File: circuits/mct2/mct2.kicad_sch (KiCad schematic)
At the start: 16 parts

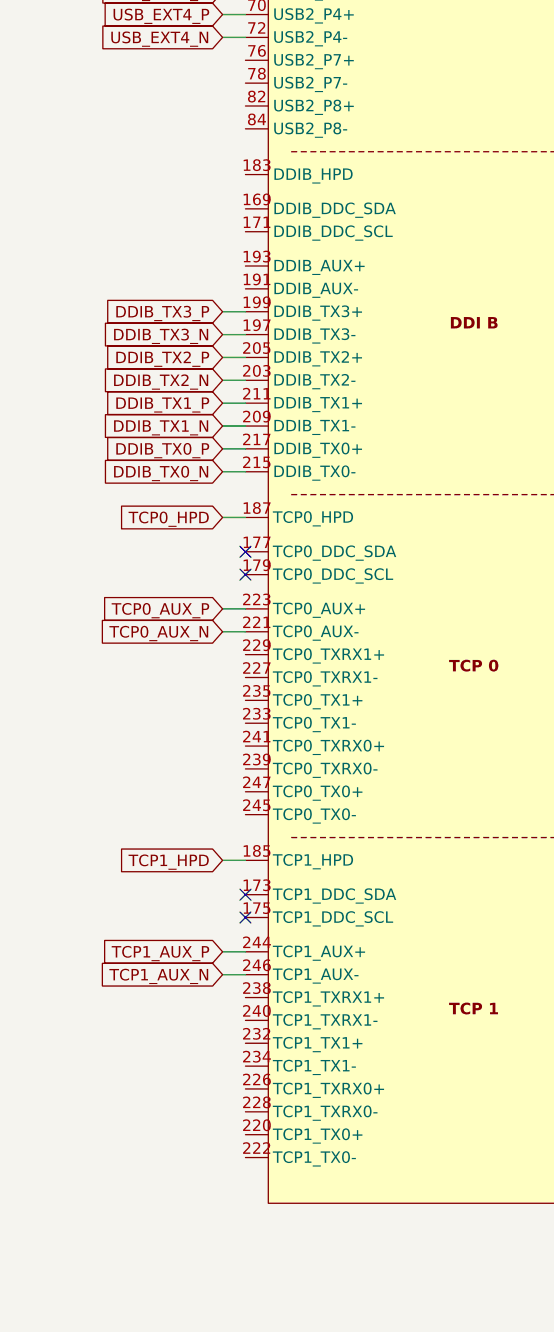
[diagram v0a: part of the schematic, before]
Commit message: Aug 14, 2024 old stuff
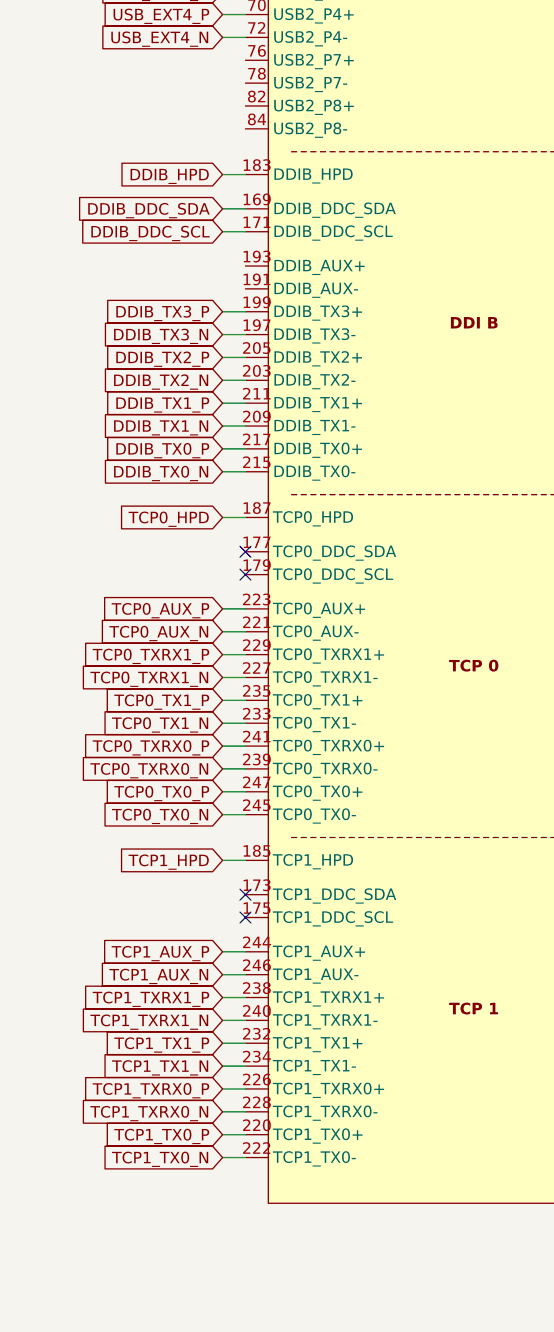
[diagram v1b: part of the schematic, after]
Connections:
- net DDIB_DDC_SDA: now reaches A1.169 (DDIB_DDC_SDA)
- net DDIB_DDC_SCL: now reaches A1.171 (DDIB_DDC_SCL)
- net DDIB_HPD: now reaches A1.183 (DDIB_HPD)
- net TCP1_TX0_P: now reaches A1.220 (TCP1_TX0+)
- net TCP1_TX0_N: now reaches A1.222 (TCP1_TX0-)
- net TCP1_TXRX0_P: now reaches A1.226 (TCP1_TXRX0+)
- net TCP0_TXRX1_N: now reaches A1.227 (TCP0_TXRX1-)
- net TCP1_TXRX0_N: now reaches A1.228 (TCP1_TXRX0-)
- net TCP0_TXRX1_P: now reaches A1.229 (TCP0_TXRX1+)
- net TCP1_TX1_P: now reaches A1.232 (TCP1_TX1+)
- net TCP0_TX1_N: now reaches A1.233 (TCP0_TX1-)
- net TCP1_TX1_N: now reaches A1.234 (TCP1_TX1-)
- net TCP0_TX1_P: now reaches A1.235 (TCP0_TX1+)
- net TCP1_TXRX1_P: now reaches A1.238 (TCP1_TXRX1+)
- net TCP0_TXRX0_N: now reaches A1.239 (TCP0_TXRX0-)
- net TCP1_TXRX1_N: now reaches A1.240 (TCP1_TXRX1-)
- net TCP0_TXRX0_P: now reaches A1.241 (TCP0_TXRX0+)
- net TCP0_TX0_N: now reaches A1.245 (TCP0_TX0-)
- net TCP0_TX0_P: now reaches A1.247 (TCP0_TX0+)
